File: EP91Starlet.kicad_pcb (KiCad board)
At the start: 2 copper layers, 116.8 x 96.5 mm, 4 parts, among them M1 Module-mega-mcu64-0.1, M2 Module-wbo-0.5, M3 Module-vr-max9924-0.1, M4 Module-knock-0.2

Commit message: more testing
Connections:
- M1 pad G: unconnected-(M1-GND-PadG) -> GND
- M1 pad N22: unconnected-(M1-V33-PadN22) -> Net-(M4-VREF)
- M1 pad S26: unconnected-(M1-IN_ADC10/EINT0_(VR_CRK)-PadS26) -> Net-(M1-IN_ADC10/EINT0_(VR_CRK))
- M1 pad W12: unconnected-(M1-CAN1H-PadW12) -> Net-(M1-CAN1H)
- M1 pad W13: unconnected-(M1-CAN1L-PadW13) -> Net-(M1-CAN1L)
- M2 pad G: unconnected-(M2-GND-PadG) -> GND
- M2 pad W3: unconnected-(M2-CANL-PadW3) -> Net-(M1-CAN1H)
- M2 pad W4: unconnected-(M2-CANH-PadW4) -> Net-(M1-CAN1L)
- M3 pad E3: unconnected-(M3-OUT-PadE3) -> Net-(M1-IN_ADC10/EINT0_(VR_CRK))
- M3 pad G: unconnected-(M3-GND-PadG) -> GND
- M4 pad E2: unconnected-(M4-GND-PadE2) -> GND
- M4 pad W2: unconnected-(M4-VREF-PadW2) -> Net-(M4-VREF)

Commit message: Fix pcb layers
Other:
- copper layers 2 -> 4

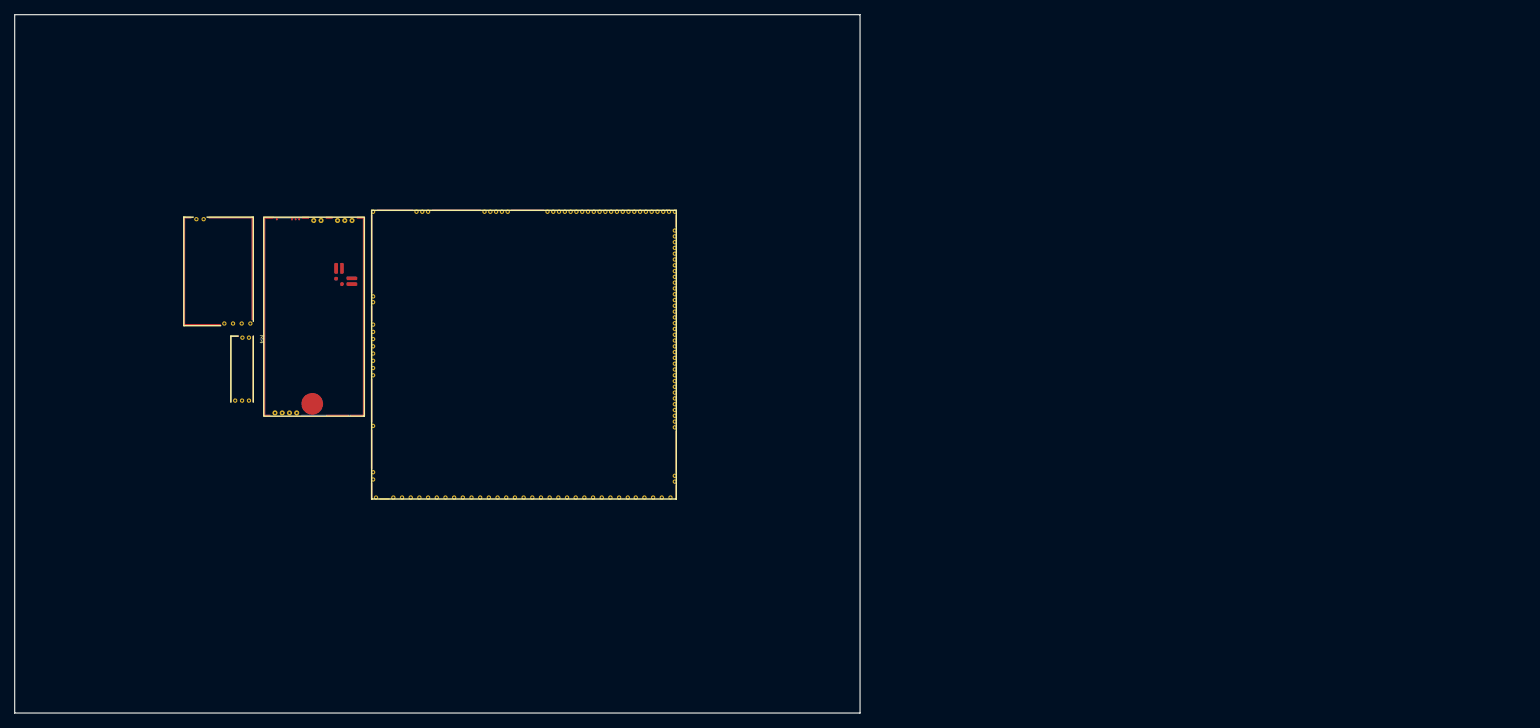
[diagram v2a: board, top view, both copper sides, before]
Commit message: 65urft7ih
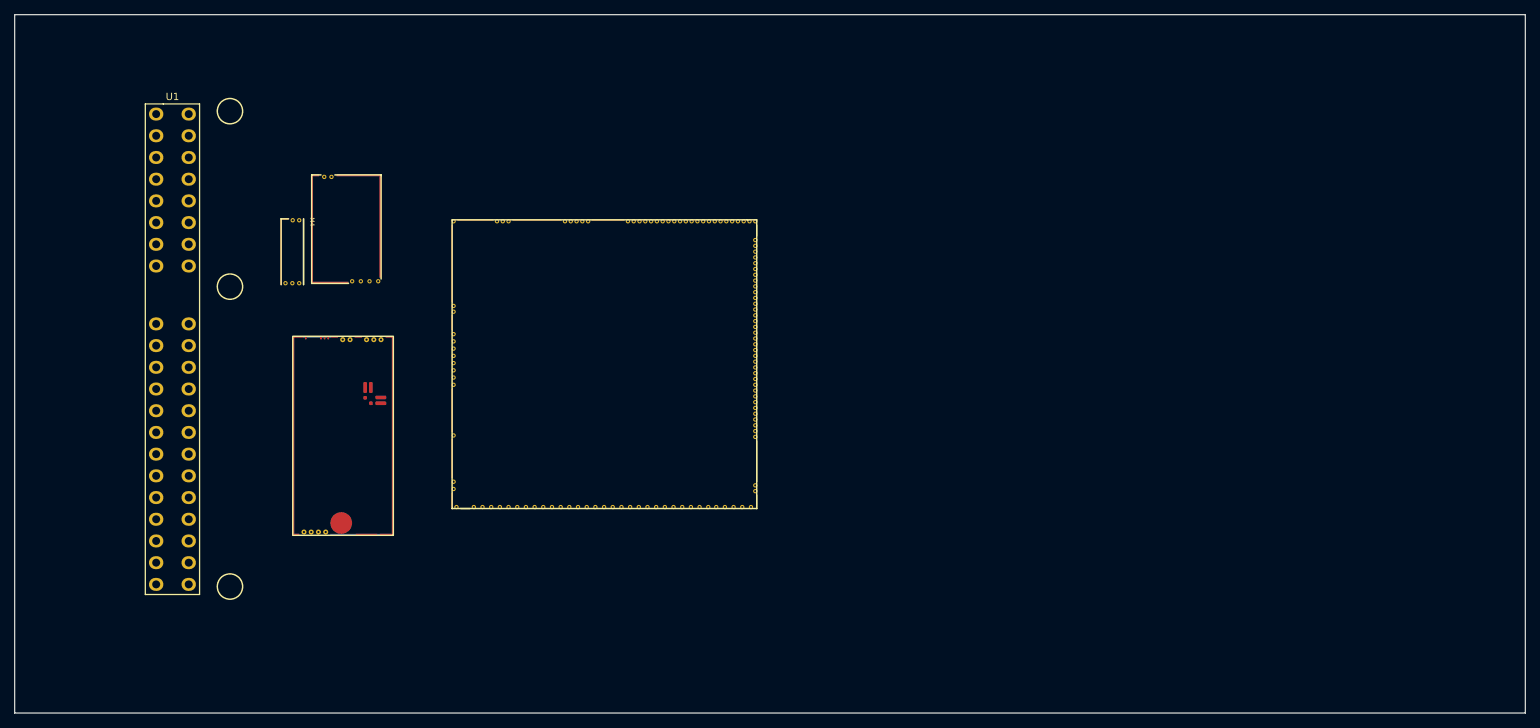
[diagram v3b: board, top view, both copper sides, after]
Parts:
- added U1: ~, EP91Starlet:4EFE ECU Connector, F.Cu at (90.4, 86.9)
- moved M3 18.6 mm to (109.5, 65.2)
- moved M4 17.6 mm to (105.3, 71.3)
- moved M2 16.9 mm to (106.9, 87.5)
- moved M1 11.2 mm to (128.9, 111.5)
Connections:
- M1 pad G: GND -> unconnected-(M1-GND-PadG)
- M1 pad W12: Net-(M1-CAN1H) -> /CAN+
- M1 pad W13: Net-(M1-CAN1L) -> /CAN-
- M2 pad G: GND -> unconnected-(M2-GND-PadG)
- M2 pad W3: Net-(M1-CAN1H) -> /CAN-
- M2 pad W4: Net-(M1-CAN1L) -> /CAN+
- M3 pad G: GND -> unconnected-(M3-GND-PadG)
- M4 pad E2: GND -> unconnected-(M4-GND-PadE2)
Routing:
- net /CAN-: track 0.00 -> 17.3 mm
- net /CAN+: track 0.00 -> 16.3 mm
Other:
- board size 116.8 x 96.5 mm -> 208.8 x 96.5 mm
